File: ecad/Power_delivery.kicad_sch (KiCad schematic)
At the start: 3 parts, among them IC2 AP2112K-3.3TRG1

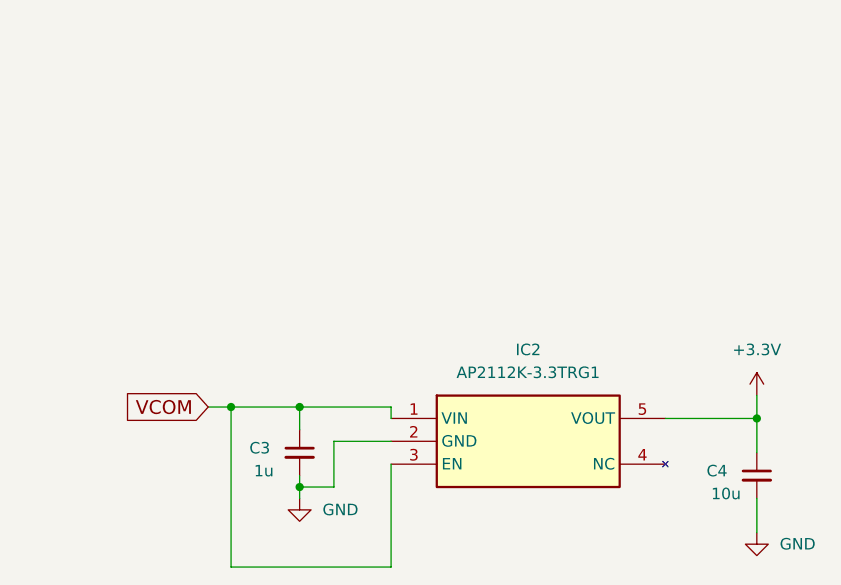
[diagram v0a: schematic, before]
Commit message: LDO change
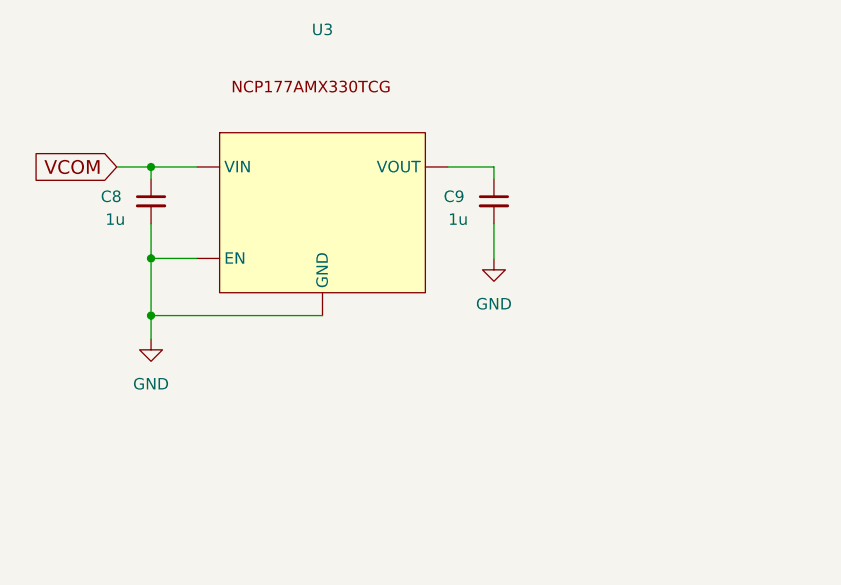
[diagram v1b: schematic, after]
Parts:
- removed C3: 1u, symbol PutRocketLab_RCL:C_Small
- removed C4: 10u, symbol PutRocketLab_RCL:C_Small
- removed IC2: AP2112K-3.3TRG1, SOT95P285X140-5N, symbol AP2112K-3_3TRG1:AP2112K-3.3TRG1
- added C8, C9: 1u, symbol PutRocketLab_RCL:C_Small
- added U3: ~, symbol NCP177AMX330TCG :NCP177AMX330TCG_
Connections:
- net GND: now also C8.2, C9.2, U3. (VOUT)
- net VCOM: now also C8.1, U3. (VOUT)
- new net: C9.1, U3. (VOUT)
